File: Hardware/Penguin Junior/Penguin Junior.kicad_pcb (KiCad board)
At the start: 4 copper layers, 58.5 x 25.4 mm, 124 parts, among them J1 Conn_02x05_SWD, J10 Conn_01x10, J11 Conn_01x10, J12 Conn_01x06_UART, J13 Conn_01x04_UART, J14 Conn_01x01, J2 Conn_02x05_SWD, J3 Micro_SD_Card_Det1, J4 Conn_01x03_Video, J5 USB_B_Micro, J6 Conn_01x03_Video, J7 Conn_01x06_UART, J8 Conn_01x04_I2C, J9 Conn_01x10, Q1 BSS138, SW1 SW_Push, U1 STM32F405RGTx, U2 BMP388, U3 BMI088, U4 MAX7456, U5 ST1S14PHR, U6 INA219AxD, U7 LDL1117_3V3, Y1 16MHz, Y2 27MHz

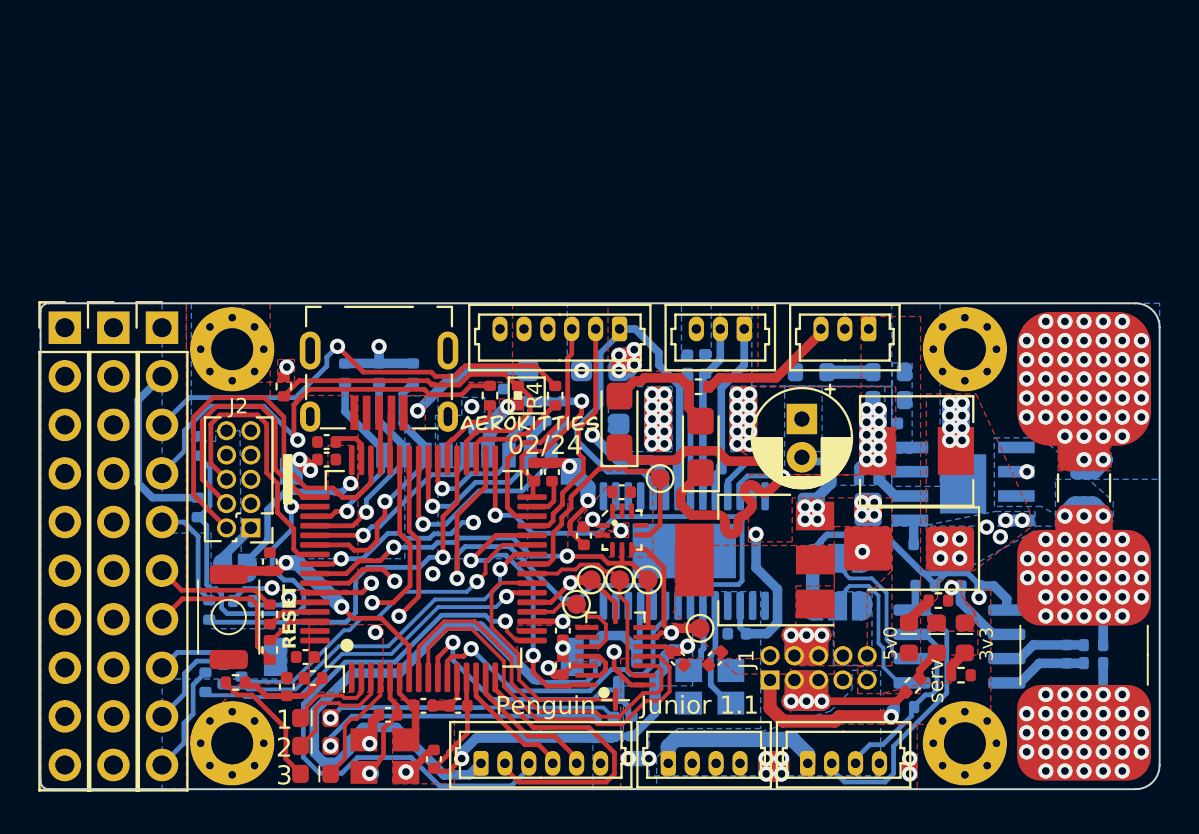
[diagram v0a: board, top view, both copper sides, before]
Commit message: Minor changes
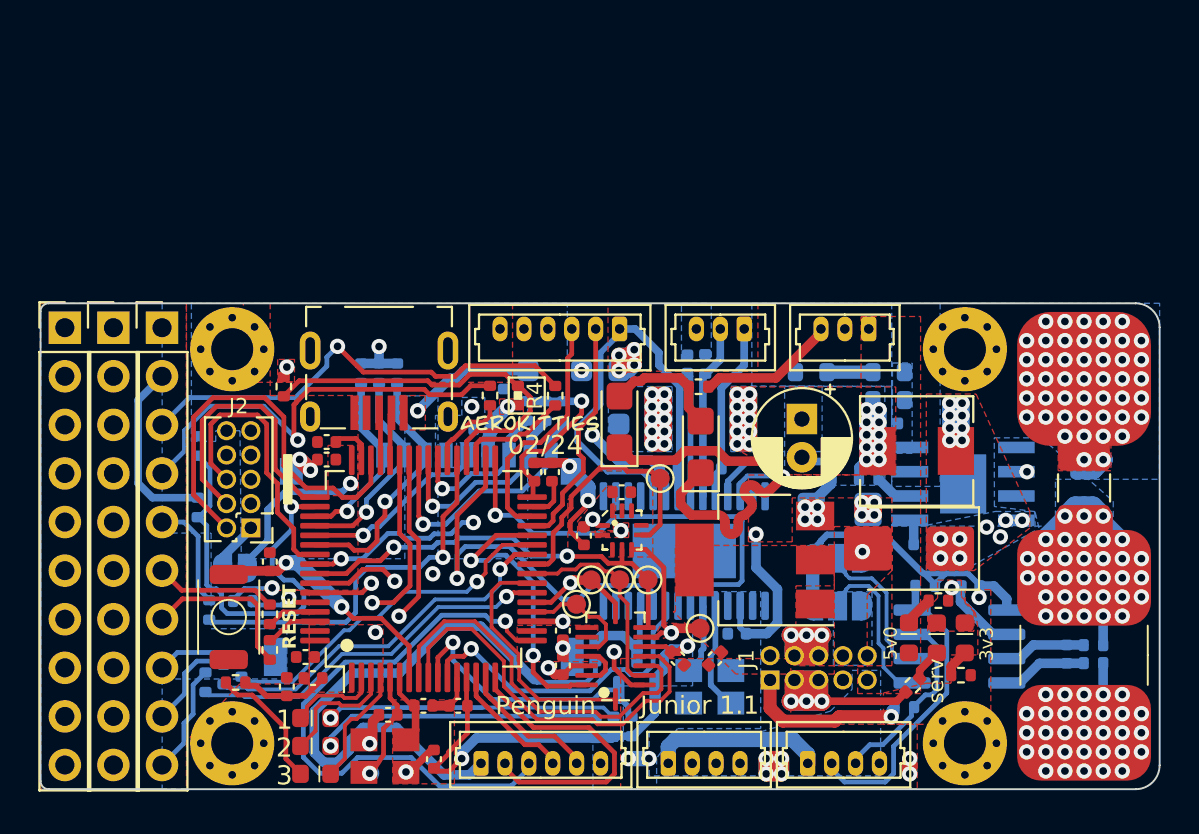
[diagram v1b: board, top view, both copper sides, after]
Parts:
- moved R16 0.83 mm to (118.7, 87.1)
- moved R14 0.83 mm to (120.5, 87.1)
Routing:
- net VDD_BUCK_6-26_IN: track 1.64 -> 92.6 mm
- net VDD_BUCK_6-26_OUT: track 9.63 -> 64.3 mm
- net GND: track 90.6 -> 113.5 mm
- net VDD_3V3: track 89.2 -> 87.6 mm
- added copper zone on B.Cu, net VDD_BUCK_6-26_IN
- added copper zone on F.Cu, net VDD_BUCK_6-26_IN
- added copper zone on In1.Cu, net VDD_BUCK_6-26_IN
- added copper zone on In2.Cu, net VDD_BUCK_6-26_IN
- added copper zone on F.Cu, net VDD_BUCK_6-26_OUT
- added copper zone on In1.Cu, net VDD_BUCK_6-26_OUT
- added copper zone on In2.Cu, net VDD_BUCK_6-26_OUT

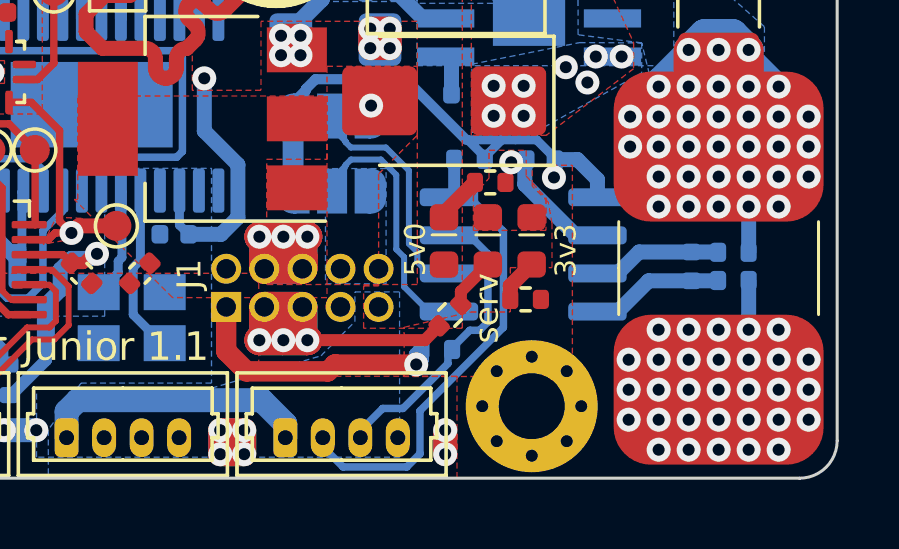
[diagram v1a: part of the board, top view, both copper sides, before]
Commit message: Updated KiCad version
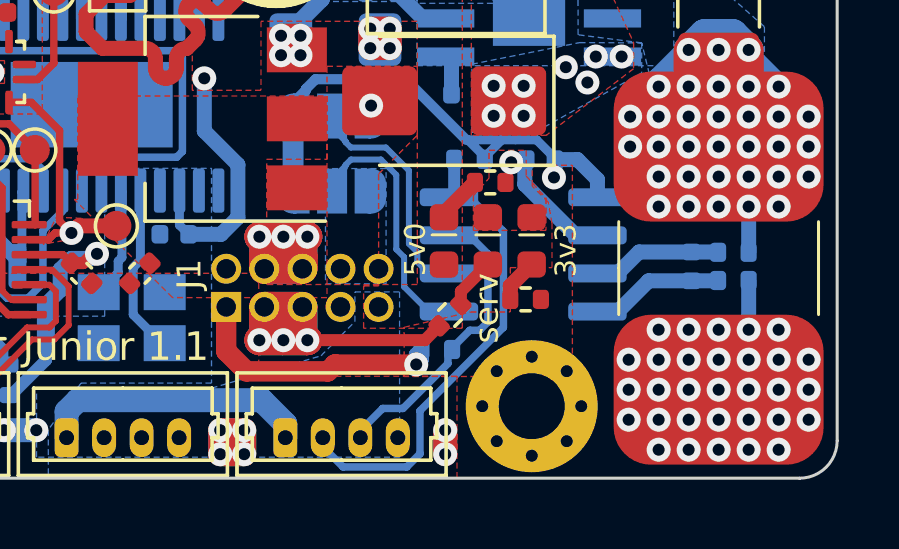
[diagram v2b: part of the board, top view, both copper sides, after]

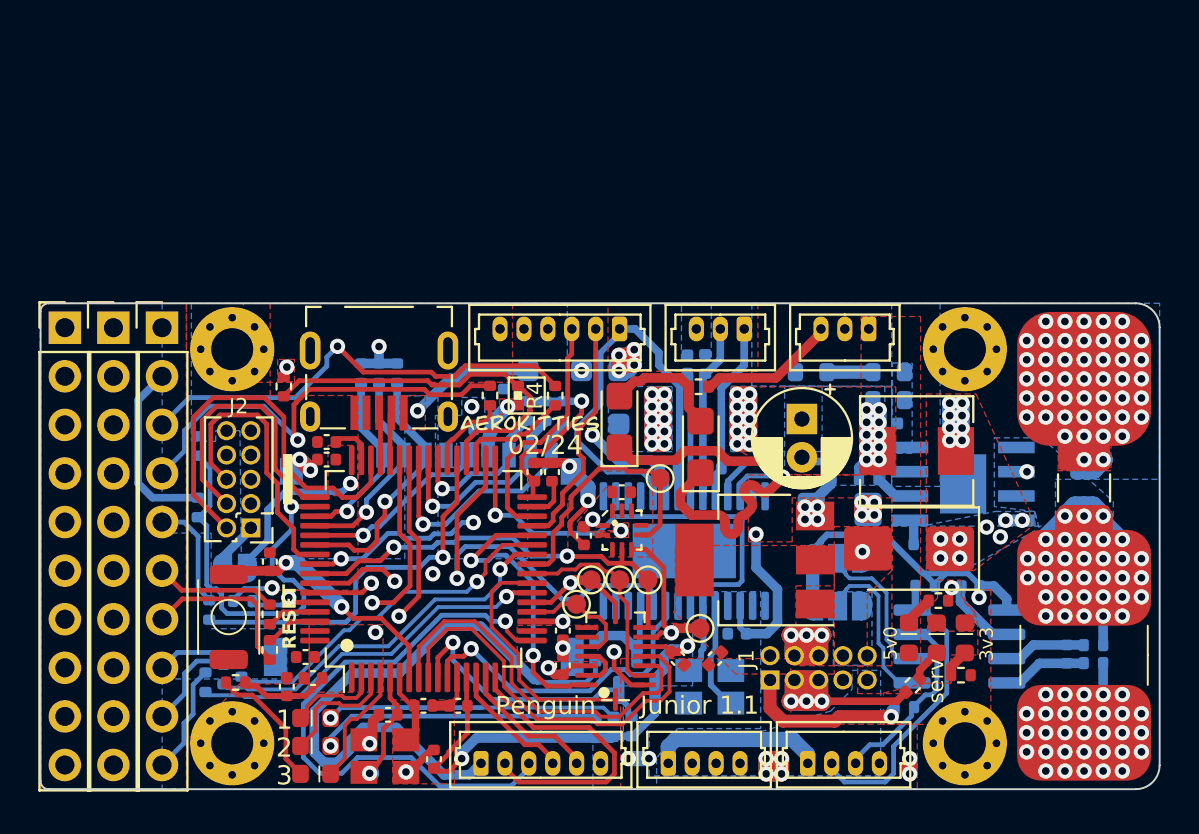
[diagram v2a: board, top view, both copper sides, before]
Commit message: Penguin Junior 1.2 prototype
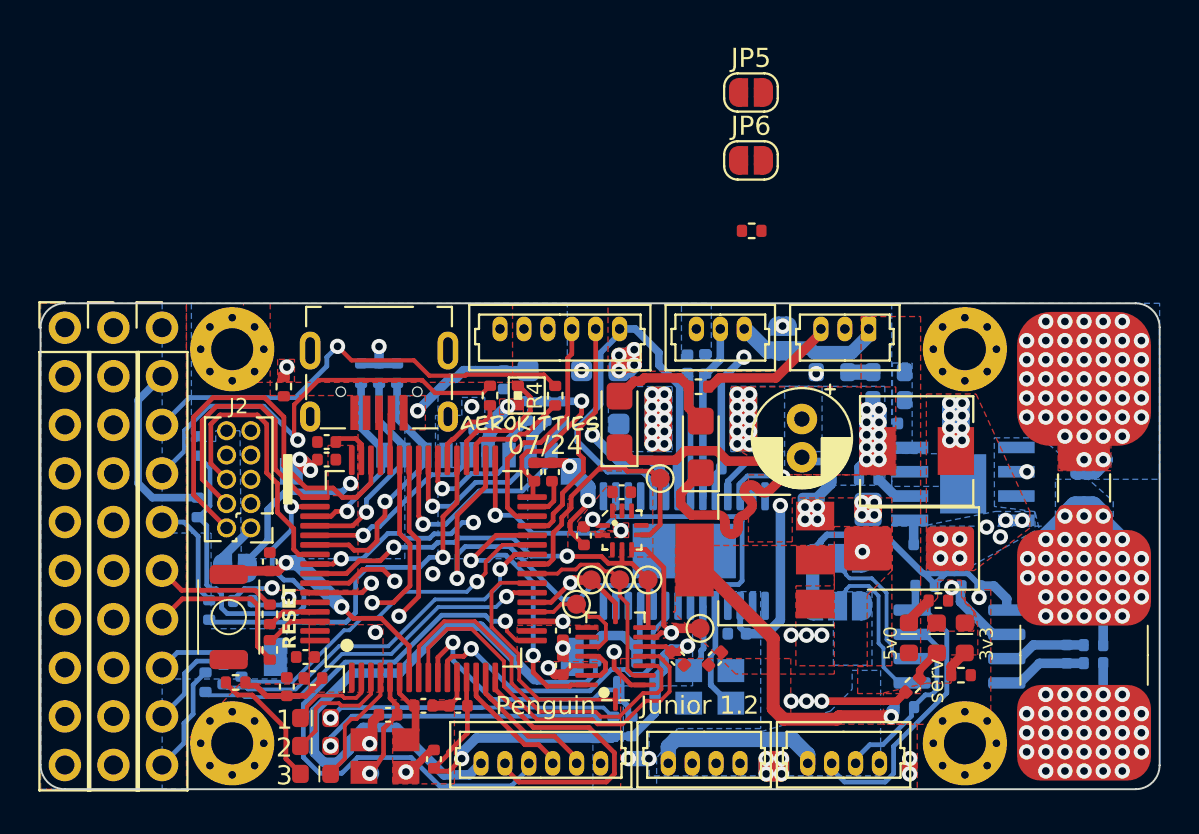
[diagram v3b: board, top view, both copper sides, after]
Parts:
- removed J1: Conn_02x05_SWD, Connector_PinHeader_1.27mm:PinHeader_2x05_P1.27mm_Vertical
- added JP4: SolderJumper_2_Open, Jumper:SolderJumper-2_P1.3mm_Open_RoundedPad1.0x1.5mm, B.Cu at (140.7, 85.3)
- added JP5: SolderJumper_2_Open, Jumper:SolderJumper-2_P1.3mm_Open_RoundedPad1.0x1.5mm, F.Cu at (139.0, 72.4)
- added JP6: SolderJumper_2_Open, Jumper:SolderJumper-2_P1.3mm_Open_RoundedPad1.0x1.5mm, F.Cu at (139.0, 76.0)
- added R39: 10K, Resistor_SMD:R_0402_1005Metric, F.Cu at (139.1, 79.7)
- moved R3 1.09 mm to (143.3, 87.1)
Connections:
- C1 pad 2: VDD_3V3 -> 3V3_JP
- C14 pad 2: VDD_3V3 -> 3V3_JP
- C15 pad 2: VDD_3V3 -> 3V3_JP
- C16 pad 1: VDD_3V3 -> 3V3_JP
- C17 pad 1: VDD_5V -> 5V0_JP
- C18 pad 1: VDD_5V -> 5V0_JP
- C19 pad 1: VDD_5V -> 5V0_JP
- C2 pad 2: VDD_3V3 -> 3V3_JP
- C24 pad 2: VDD_3V3 -> 3V3_JP
- C27 pad 1: VDD_3V3 -> 3V3_JP
- C3 pad 2: VDD_3V3 -> 3V3_JP
- C35 pad 1: VDD_3V3 -> 3V3_JP
- C4 pad 2: VDD_3V3 -> 3V3_JP
- C5 pad 2: VDD_3V3 -> 3V3_JP
- C6 pad 2: VDD_3V3 -> 3V3_JP
- C7 pad 2: VDD_3V3 -> 3V3_JP
- C8 pad 2: VDD_3V3 -> 3V3_JP
- D7 pad 2: VDD_5V -> 5V0_JP
- J12 pad 1: VDD_5V -> 5V0_JP
- J13 pad 1: VDD_5V -> 5V0_JP
- J3 pad 4: VDD_3V3 -> 3V3_JP
- J4 pad 1: VDD_5V -> Net-(J4-Pin_1)
- J6 pad 1: VDD_5V -> Net-(J4-Pin_1)
- J7 pad 1: VDD_5V -> 5V0_JP
- J8 pad 1: VDD_5V -> 5V0_JP
- JP1 pad 1: VDD_3V3 -> 3V3_JP
- JP2 pad 3: VDD_3V3 -> 3V3_JP
- JP3 pad 3: VDD_3V3 -> 3V3_JP
- Q1 pad 1: VDD_3V3 -> 3V3_JP
- R10 pad 1: BOOT0 -> Net-(JP6-A)
- R10 pad 2: Net-(J1-Pin_7) -> GND
- R11 pad 1: VDD_3V3 -> 3V3_JP
- R12 pad 1: VDD_3V3 -> 3V3_JP
- R13 pad 1: VDD_3V3 -> 3V3_JP
- R14 pad 1: VDD_3V3 -> 3V3_JP
- R15 pad 1: VDD_3V3 -> 3V3_JP
- R16 pad 2: VDD_3V3 -> 3V3_JP
- R20 pad 2: VDD_3V3 -> 3V3_JP
- R21 pad 2: VDD_3V3 -> 3V3_JP
- R33 pad 2: VDD_3V3 -> 3V3_JP
- R34 pad 2: VDD_3V3 -> 3V3_JP
- R35 pad 2: VDD_3V3 -> 3V3_JP
- R38 pad 1: VDD_3V3 -> 3V3_JP
- R7 pad 1: VDD_3V3 -> 3V3_JP
- R8 pad 1: VDD_5V -> 5V0_JP
- U1 pad 1: VDD_3V3 -> 3V3_JP
- U1 pad 13: VDD_3V3 -> 3V3_JP
- U1 pad 19: VDD_3V3 -> 3V3_JP
- U1 pad 32: VDD_3V3 -> 3V3_JP
- U1 pad 48: VDD_3V3 -> 3V3_JP
- U1 pad 64: VDD_3V3 -> 3V3_JP
- U2 pad 1: VDD_3V3 -> 3V3_JP
- U2 pad 10: VDD_3V3 -> 3V3_JP
- U3 pad 11: VDD_3V3 -> 3V3_JP
- U3 pad 3: VDD_3V3 -> 3V3_JP
- U4 pad 19: VDD_5V -> 5V0_JP
- U4 pad 21: VDD_5V -> 5V0_JP
- U4 pad 24: VDD_5V -> 5V0_JP
- U4 pad 3: VDD_5V -> 5V0_JP
- U6 pad 5: VDD_3V3 -> 3V3_JP
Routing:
- net 5V0_JP: track 28.1 -> 123.4 mm, vias 9 -> 12
- net 3V3_JP: track 0.01 -> 95.3 mm, vias 0 -> 12
- net VDD_5V: track 93.0 -> 0.00 mm, vias 1 -> 0
- net VDD_3V3: track 87.6 -> 0.00 mm, vias 12 -> 0
- net Net-(J1-Pin_7): track 38.9 -> 0.00 mm, vias 2 -> 0
- net GND: track 113.5 -> 152.4 mm, vias 66 -> 69
- net VDD_5V_SERVO: track 27.7 -> 4.59 mm
- net 5V0_SERVO_JP: track 46.8 -> 26.0 mm
- net TM12_CH2/ADC1_EXTI15: track 19.8 -> 6.60 mm
- net Net-(J4-Pin_1): track 0.00 -> 7.81 mm
- net Net-(R2-Pad1): track 2.40 -> 1.31 mm
- added copper zone on B.Cu, net 3V3_JP
- added copper zone on In1.Cu, net 3V3_JP
- added copper zone on In2.Cu, net 3V3_JP
- added copper zone on B.Cu, net 5V0_JP
- added copper zone on F.Cu, net 5V0_JP
- removed copper zone on B.Cu, net VDD_3V3
- removed copper zone on F.Cu, net VDD_3V3
- removed copper zone on In1.Cu, net VDD_3V3
- removed copper zone on In2.Cu, net VDD_3V3
- removed copper zone on B.Cu, net VDD_5V
- removed copper zone on F.Cu, net VDD_5V
- removed copper zone on In2.Cu, net VDD_5V
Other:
- outline, holes or cut-outs redrawn
- board text added: "07/24"
- board text added: "Junior 1.2"
- board text removed: "02/24"
- board text removed: "Junior 1.1"
- board text removed: "boot0"

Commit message: Update Penguin concept
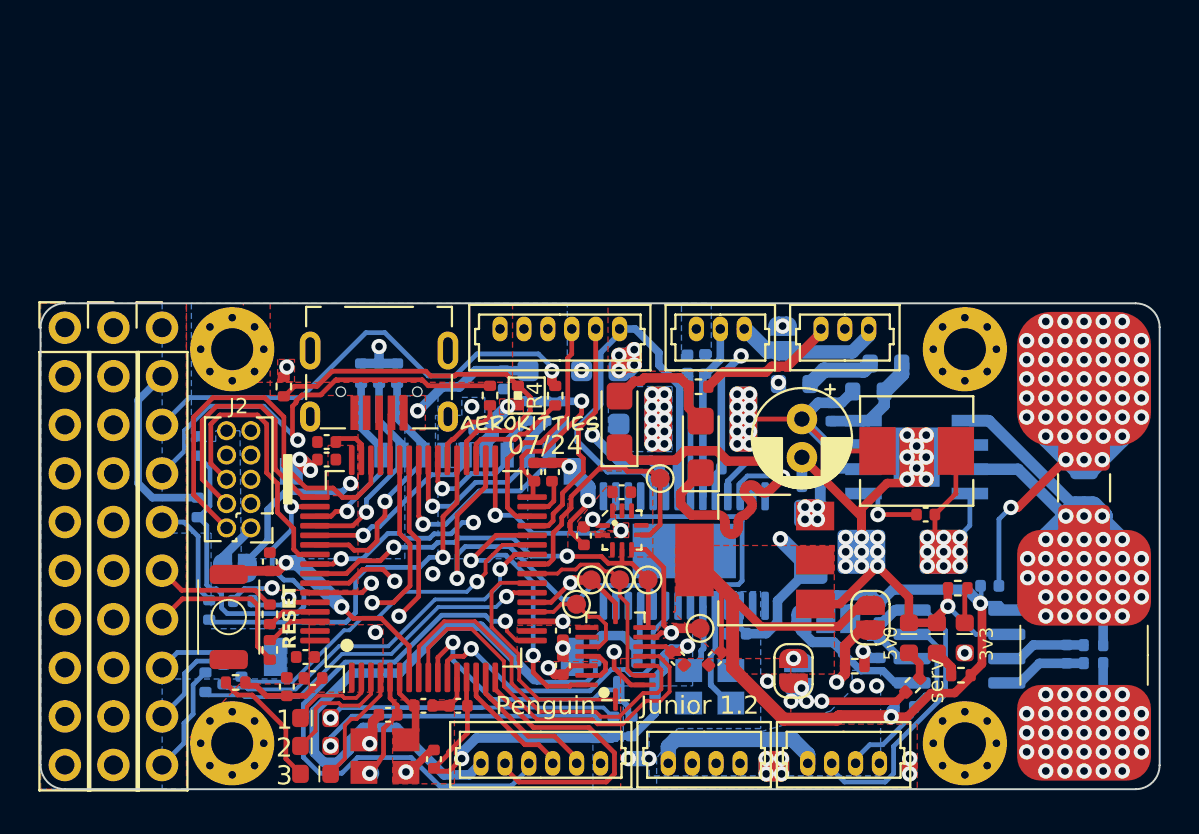
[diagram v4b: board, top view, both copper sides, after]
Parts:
- added R40: 10K, Resistor_SMD:R_0402_1005Metric, B.Cu at (144.4, 101.7)
- added R41: 10K, Resistor_SMD:R_0402_1005Metric, B.Cu at (145.8, 101.5)
- C26, R10: moved to F.Cu
- D5, R39: moved to B.Cu
- J3: footprint sd:TF01A -> sd:TF01A-NEW
- JP2: value SolderJumper_3_Open -> SolderJumper_2_Open; footprint Jumper:SolderJumper-3_P1.3mm_Open_RoundedPad1.0x1.5mm_NumberLabels -> Jumper:SolderJumper-2_P1.3mm_Open_RoundedPad1.0x1.5mm
- moved R39 32.9 mm to (112.5, 99.0), turned to 180 degrees
- moved R10 32.2 mm to (144.5, 102.4), turned to 0 degrees
- moved JP5 30.3 mm to (141.3, 102.7), turned to -90 degrees
- moved JP6 24.7 mm to (145.3, 99.9), turned to 90 degrees
- moved JP2 4.14 mm to (141.5, 102.9), turned to -90 degrees
- moved JP3 3.22 mm to (143.0, 100.0)
- moved C32 3.05 mm to (143.2, 89.1), turned to 90 degrees
- moved D7 2.92 mm to (150.2, 101.0)
- moved U5 2.80 mm to (147.7, 91.5)
- moved R21 2.76 mm to (145.8, 99.6), turned to 90 degrees
- moved F2 2.27 mm to (142.2, 95.9), turned to 90 degrees
- moved R32 2.23 mm to (143.2, 91.6), turned to 90 degrees
- moved R3 2.07 mm to (141.3, 87.7)
- moved C26 1.56 mm to (148.2, 94.5)
- moved D9 1.46 mm to (148.8, 101.0)
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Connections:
- JP2 pad 1: GND -> 5V0_SERVO_JP
- JP2 pad 2: Net-(JP2-C) -> VDD_5V_SERVO
- JP3 pad 1: GND -> Net-(JP3-A)
- JP3 pad 2: Net-(JP3-C) -> 3V3_JP
- JP3 pad 3: 3V3_JP -> Net-(JP3-B)
- U6 pad 1: Net-(JP2-C) -> Net-(JP3-B)
- U6 pad 2: Net-(JP3-C) -> Net-(JP3-A)
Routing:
- net Net-(JP6-A): track 0.00 -> 42.4 mm, vias 0 -> 3
- net GND: track 152.4 -> 192.8 mm, vias 69 -> 86
- net 3V3_JP: track 95.3 -> 115.5 mm, vias 12 -> 13
- net TM12_CH2/ADC1_EXTI15: track 6.60 -> 19.8 mm
- net 5V0_JP: track 123.4 -> 112.8 mm, vias 12 -> 11
- net VDD_BUCK_6-26_OUT: track 64.3 -> 74.4 mm
- net Net-(JP2-C): track 8.71 -> 0.00 mm
- net Net-(JP3-C): track 7.94 -> 0.00 mm
- net Net-(JP3-B): track 0.00 -> 7.59 mm
- net Net-(D5-K): track 27.6 -> 33.8 mm, vias 16 -> 9
- net Net-(U5-FB): track 0.00 -> 5.67 mm
- net Net-(JP3-A): track 0.00 -> 4.07 mm
- net Net-(U5-BOOT): track 1.34 -> 3.87 mm, vias 0 -> 1
- net Net-(R2-Pad1): track 1.31 -> 3.59 mm
- net Net-(J9-Pin_3): track 23.4 -> 25.1 mm
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- removed copper zone on B.Cu, net Net-(D5-K)
- removed copper zone on F.Cu, net Net-(D5-K)
- removed copper zone on In2.Cu, net Net-(D5-K)
- removed copper zone on B.Cu, net Net-(U5-FB)
- removed copper zone on B.Cu, net VDD_BUCK_5V
- removed copper zone on F.Cu, net VDD_BUCK_5V
- removed copper zone on In2.Cu, net VDD_BUCK_5V
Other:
- board text removed: "0"
- board text removed: "JP2"
- board text removed: "JP3"
